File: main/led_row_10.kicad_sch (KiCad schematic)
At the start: 30 parts

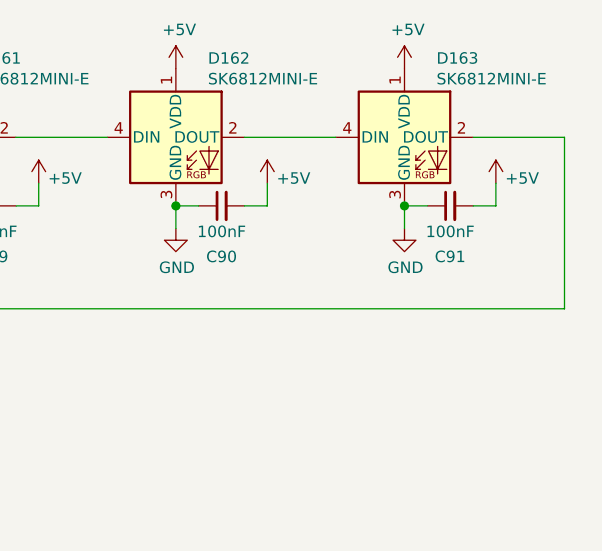
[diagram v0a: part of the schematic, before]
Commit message: Start placing diodes
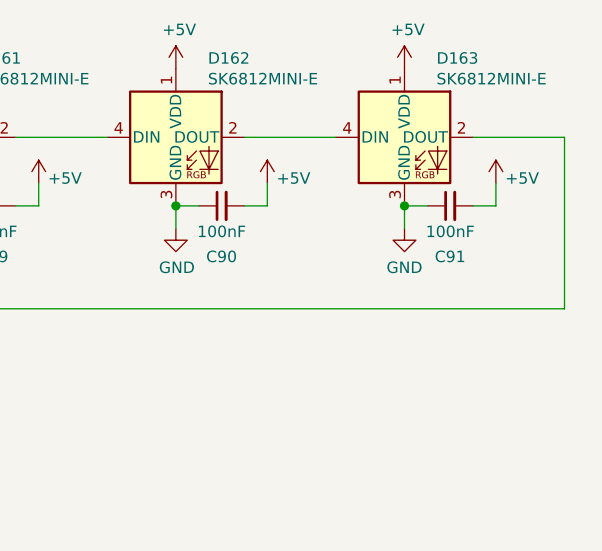
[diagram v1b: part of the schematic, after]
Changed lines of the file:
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@@
   )
   (symbol (lib_id "power:GND") (at 262.89 36.83 0) (unit 1)
-    (in_bom yes) (on_board yes)
-    (property "Reference" "#PWR0273" (id 0) (at 262.89 43.18 0)
-      (effects (font (size 1.27 1.27)) hide)
-    )
-    (property "Value" "GND" (id 1) (at 263.0043 41.1544 0))
+    (in_bom yes) (on_board yes) (fields_autoplaced)
+    (property "Reference" "#PWR053" (id 0) (at 262.89 43.18 0)
+      (effects (font (size 1.27 1.27)) hide)
+    )
+    (property "Value" "GND" (id 1) (at 262.89 41.1544 0))
     (property "Footprint" "" (id 2) (at 262.89 36.83 0)
       (effects (font (size 1.27 1.27)) hide)
@@
     (pin "4")
   )
-  (symbol (lib_id "chonc60:SK6812MINI-E") (at 34.29 26.67 0) (unit 1)
+  (symbol (lib_name "chonc60:SK6812MINI-E_14") (lib_id "chonc60:SK6812MINI-E") (at 34.29 26.67 0) (unit 1)
     (in_bom yes) (on_board yes)
     (property "Reference" "D154" (id 0) (at 37.8461 17.9006 0)
@@
     (pin "4")
   )
-  (symbol (lib_id "chonc60:SK6812MINI-E") (at 58.42 63.5 0) (unit 1)
+  (symbol (lib_name "chonc60:SK6812MINI-E_12") (lib_id "chonc60:SK6812MINI-E") (at 58.42 63.5 0) (unit 1)
     (in_bom yes) (on_board yes)
     (property "Reference" "D165" (id 0) (at 61.9761 54.7306 0)
@@
     (pin "4")
   )
-  (symbol (lib_id "chonc60:SK6812MINI-E") (at 59.69 26.67 0) (unit 1)
+  (symbol (lib_name "chonc60:SK6812MINI-E_11") (lib_id "chonc60:SK6812MINI-E") (at 59.69 26.67 0) (unit 1)
     (in_bom yes) (on_board yes)
     (property "Reference" "D155" (id 0) (at 63.2461 17.9006 0)
@@
     (pin "4")
   )
-  (symbol (lib_id "chonc60:SK6812MINI-E") (at 83.82 63.5 0) (unit 1)
+  (symbol (lib_name "chonc60:SK6812MINI-E_13") (lib_id "chonc60:SK6812MINI-E") (at 83.82 63.5 0) (unit 1)
     (in_bom yes) (on_board yes)
     (property "Reference" "D166" (id 0) (at 87.3761 54.7306 0)
@@
     (pin "4")
   )
-  (symbol (lib_id "chonc60:SK6812MINI-E") (at 85.09 26.67 0) (unit 1)
+  (symbol (lib_name "chonc60:SK6812MINI-E_10") (lib_id "chonc60:SK6812MINI-E") (at 85.09 26.67 0) (unit 1)
     (in_bom yes) (on_board yes)
     (property "Reference" "D156" (id 0) (at 88.6461 17.9006 0)
@@
     (pin "4")
   )
-  (symbol (lib_id "chonc60:SK6812MINI-E") (at 109.22 63.5 0) (unit 1)
+  (symbol (lib_name "chonc60:SK6812MINI-E_2") (lib_id "chonc60:SK6812MINI-E") (at 109.22 63.5 0) (unit 1)
     (in_bom yes) (on_board yes)
     (property "Reference" "D167" (id 0) (at 112.7761 54.7306 0)
@@
     (pin "4")
   )
-  (symbol (lib_id "chonc60:SK6812MINI-E") (at 110.49 26.67 0) (unit 1)
+  (symbol (lib_name "chonc60:SK6812MINI-E_7") (lib_id "chonc60:SK6812MINI-E") (at 110.49 26.67 0) (unit 1)
     (in_bom yes) (on_board yes)
     (property "Reference" "D157" (id 0) (at 114.0461 17.9006 0)
@@
     (pin "4")
   )
-  (symbol (lib_id "chonc60:SK6812MINI-E") (at 135.89 26.67 0) (unit 1)
+  (symbol (lib_name "chonc60:SK6812MINI-E_8") (lib_id "chonc60:SK6812MINI-E") (at 135.89 26.67 0) (unit 1)
     (in_bom yes) (on_board yes)
     (property "Reference" "D158" (id 0) (at 139.4461 17.9006 0)
@@
     (pin "4")
   )
-  (symbol (lib_id "chonc60:SK6812MINI-E") (at 135.89 63.5 0) (unit 1)
+  (symbol (lib_name "chonc60:SK6812MINI-E_1") (lib_id "chonc60:SK6812MINI-E") (at 135.89 63.5 0) (unit 1)
     (in_bom yes) (on_board yes)
     (property "Reference" "D168" (id 0) (at 139.4461 54.7306 0)
@@
     (pin "4")
   )
-  (symbol (lib_id "chonc60:SK6812MINI-E") (at 161.29 26.67 0) (unit 1)
+  (symbol (lib_name "chonc60:SK6812MINI-E_6") (lib_id "chonc60:SK6812MINI-E") (at 161.29 26.67 0) (unit 1)
     (in_bom yes) (on_board yes)
     (property "Reference" "D159" (id 0) (at 164.8461 17.9006 0)
@@
     (pin "4")
   )
-  (symbol (lib_id "chonc60:SK6812MINI-E") (at 186.69 26.67 0) (unit 1)
+  (symbol (lib_name "chonc60:SK6812MINI-E_9") (lib_id "chonc60:SK6812MINI-E") (at 186.69 26.67 0) (unit 1)
     (in_bom yes) (on_board yes)
     (property "Reference" "D160" (id 0) (at 190.2461 17.9006 0)
@@
     (pin "4")
   )
-  (symbol (lib_id "chonc60:SK6812MINI-E") (at 212.09 26.67 0) (unit 1)
+  (symbol (lib_name "chonc60:SK6812MINI-E_3") (lib_id "chonc60:SK6812MINI-E") (at 212.09 26.67 0) (unit 1)
     (in_bom yes) (on_board yes)
     (property "Reference" "D161" (id 0) (at 215.6461 17.9006 0)
@@
     (pin "4")
   )
-  (symbol (lib_id "chonc60:SK6812MINI-E") (at 237.49 26.67 0) (unit 1)
+  (symbol (lib_name "chonc60:SK6812MINI-E_5") (lib_id "chonc60:SK6812MINI-E") (at 237.49 26.67 0) (unit 1)
     (in_bom yes) (on_board yes)
     (property "Reference" "D162" (id 0) (at 241.0461 17.9006 0)
@@
     (pin "4")
   )
-  (symbol (lib_id "chonc60:SK6812MINI-E") (at 262.89 26.67 0) (unit 1)
+  (symbol (lib_name "chonc60:SK6812MINI-E_4") (lib_id "chonc60:SK6812MINI-E") (at 262.89 26.67 0) (unit 1)
     (in_bom yes) (on_board yes)
     (property "Reference" "D163" (id 0) (at 266.4461 17.9006 0)
